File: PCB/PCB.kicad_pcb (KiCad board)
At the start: 2 copper layers, 22.8 x 29.9 mm, 5 parts

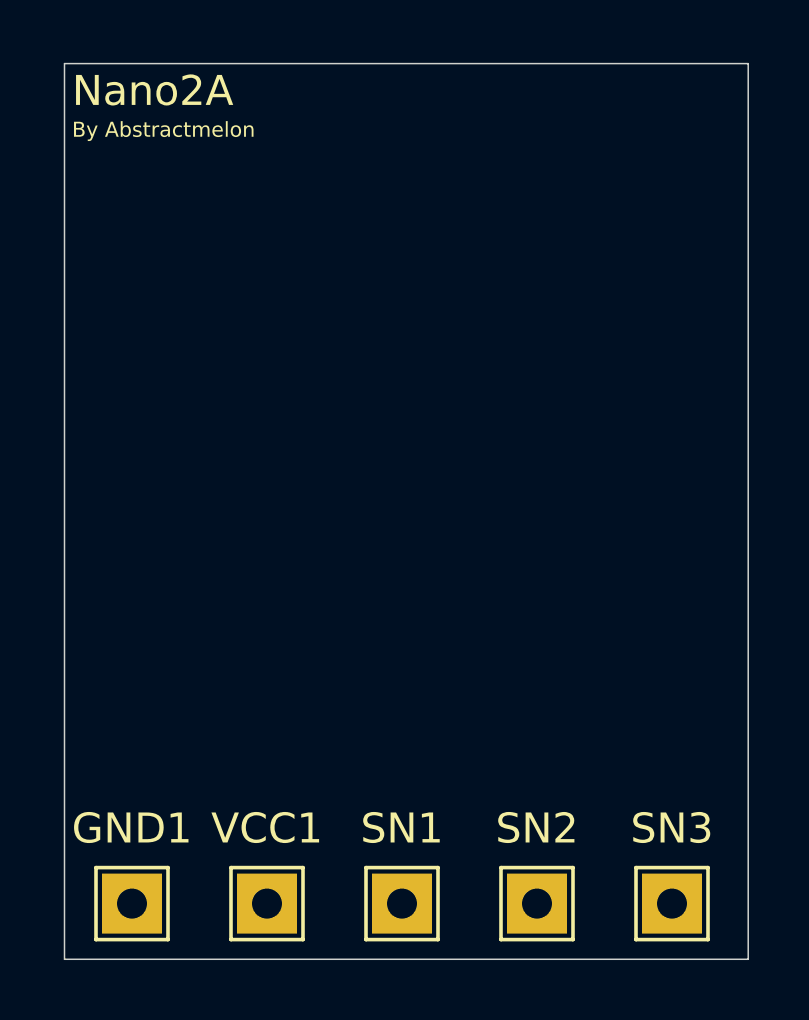
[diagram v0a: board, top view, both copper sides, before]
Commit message: feat: add components
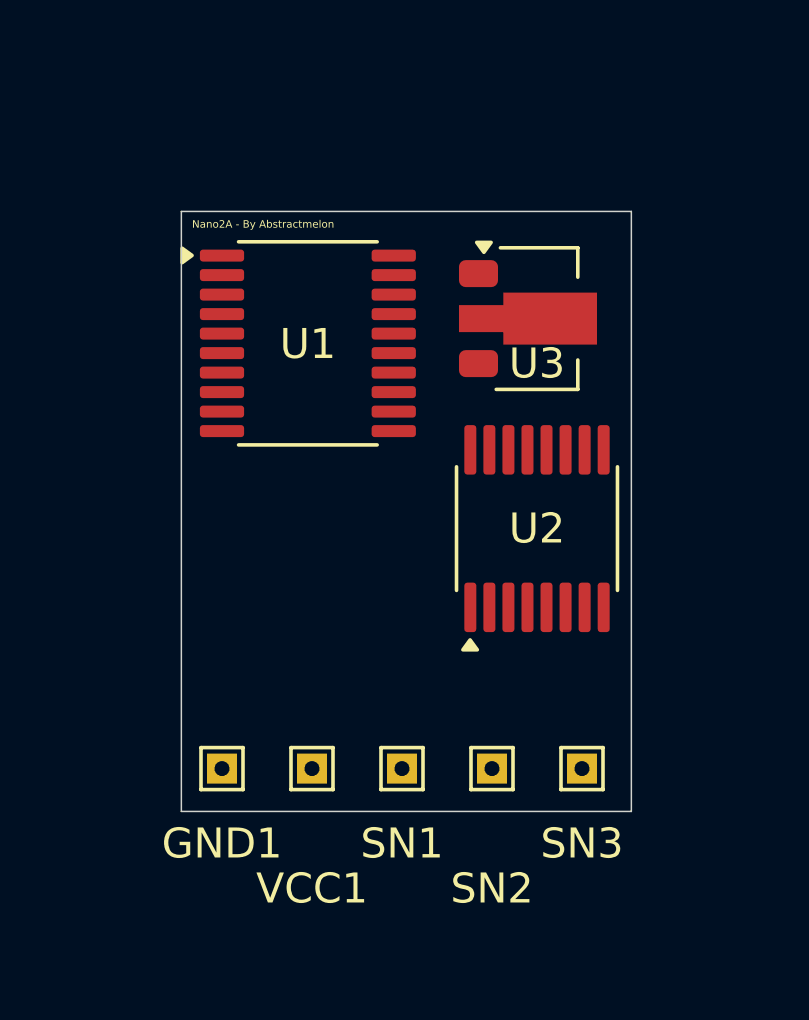
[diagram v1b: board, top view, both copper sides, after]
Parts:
- added U1: STM32G031F6P6, Package_SO:TSSOP-20_4.4x6.5mm_P0.65mm, F.Cu at (157.9, 69.3)
- added U2: XN297L, Package_SO:SSOP-16_3.9x4.9mm_P0.635mm, F.Cu at (165.5, 75.5)
- added U3: HT7333-3.3V, Package_TO_SOT_SMD:SOT-89-3, F.Cu at (165.5, 68.5)
- GND1, SN1, SN2, SN3, VCC1: footprint TestPoint:TestPoint_THTPad_2.0x2.0mm_Drill1.0mm -> TestPoint:TestPoint_THTPad_1.0x1.0mm_Drill0.5mm
- moved GND1 5.41 mm to (155.0, 83.5)
- moved SN3 5.41 mm to (167.0, 83.5)
- moved SN2 4.74 mm to (164.0, 83.5)
- moved VCC1 4.74 mm to (158.0, 83.5)
- moved SN1 4.50 mm to (161.0, 83.5)
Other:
- board size 22.8 x 29.9 mm -> 15 x 20 mm
- board text added: "Nano2A - By Abstractmelon"
- board text removed: "By Abstractmelon"
- board text removed: "Nano2A"

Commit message: feat: added all components
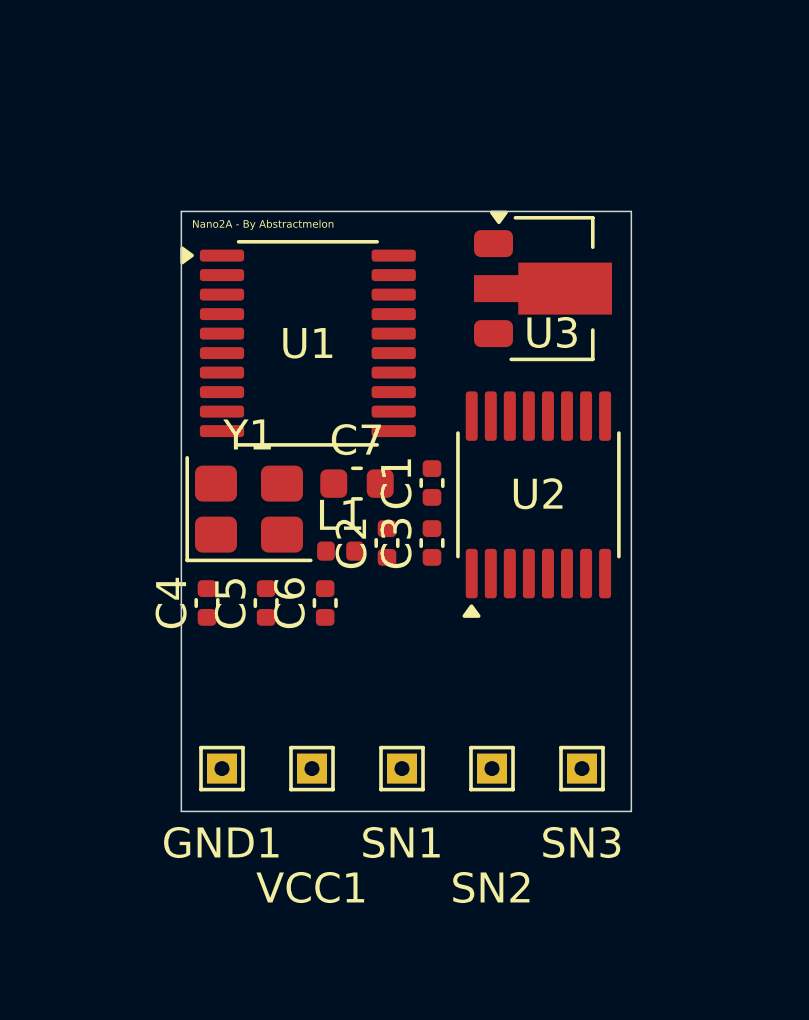
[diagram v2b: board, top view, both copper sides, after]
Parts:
- added C1: C, Capacitor_SMD:C_0402_1005Metric, F.Cu at (162.0, 74.0)
- added C2: C, Capacitor_SMD:C_0402_1005Metric, F.Cu at (160.5, 76.0)
- added C3: C, Capacitor_SMD:C_0402_1005Metric, F.Cu at (162.0, 76.0)
- added C4: C, Capacitor_SMD:C_0402_1005Metric, F.Cu at (154.5, 78.0)
- added C5: C, Capacitor_SMD:C_0402_1005Metric, F.Cu at (156.5, 78.0)
- added C6: C, Capacitor_SMD:C_0402_1005Metric, F.Cu at (158.4, 78.0)
- added C7: C, Capacitor_SMD:C_0603_1608Metric, F.Cu at (159.5, 74.0)
- added L1: L, Inductor_SMD:L_0402_1005Metric, F.Cu at (158.9, 76.2)
- added Y1: Crystal, Crystal:Crystal_SMD_3225-4Pin_3.2x2.5mm, F.Cu at (155.9, 74.8)
- moved U2 1.13 mm to (165.5, 74.4)
- moved U3 1.12 mm to (166.0, 67.5)
